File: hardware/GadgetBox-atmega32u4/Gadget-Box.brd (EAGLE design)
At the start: 93.5 x 53.5 mm, 44 parts, among them U1 MCP73831T-2ACI/OT, U2 AP2112-3.3, U3 ATMEGA32U4-XUAU, U4 ATMEGA32U4-XUMU, X1 CRYSTAL-0500290P1, X100 JSTPH

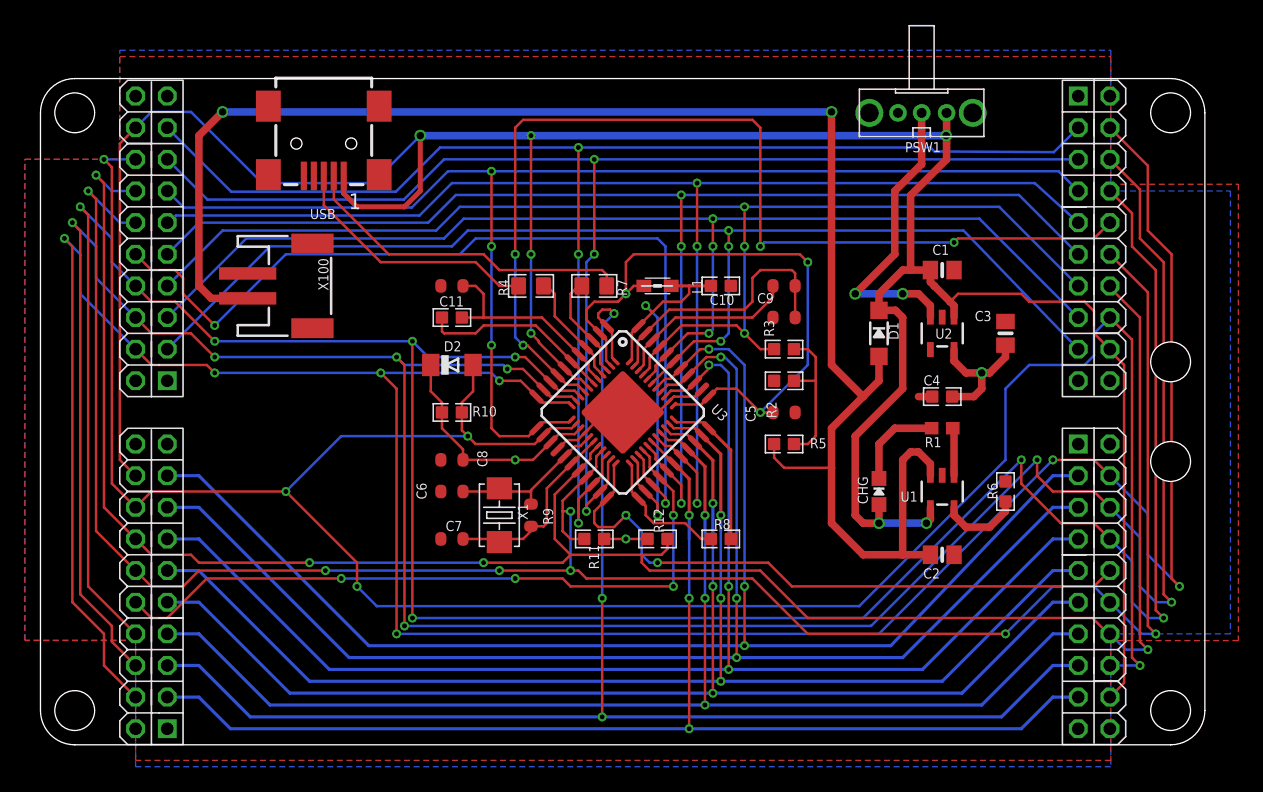
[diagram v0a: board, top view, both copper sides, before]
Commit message: cleaned up drc
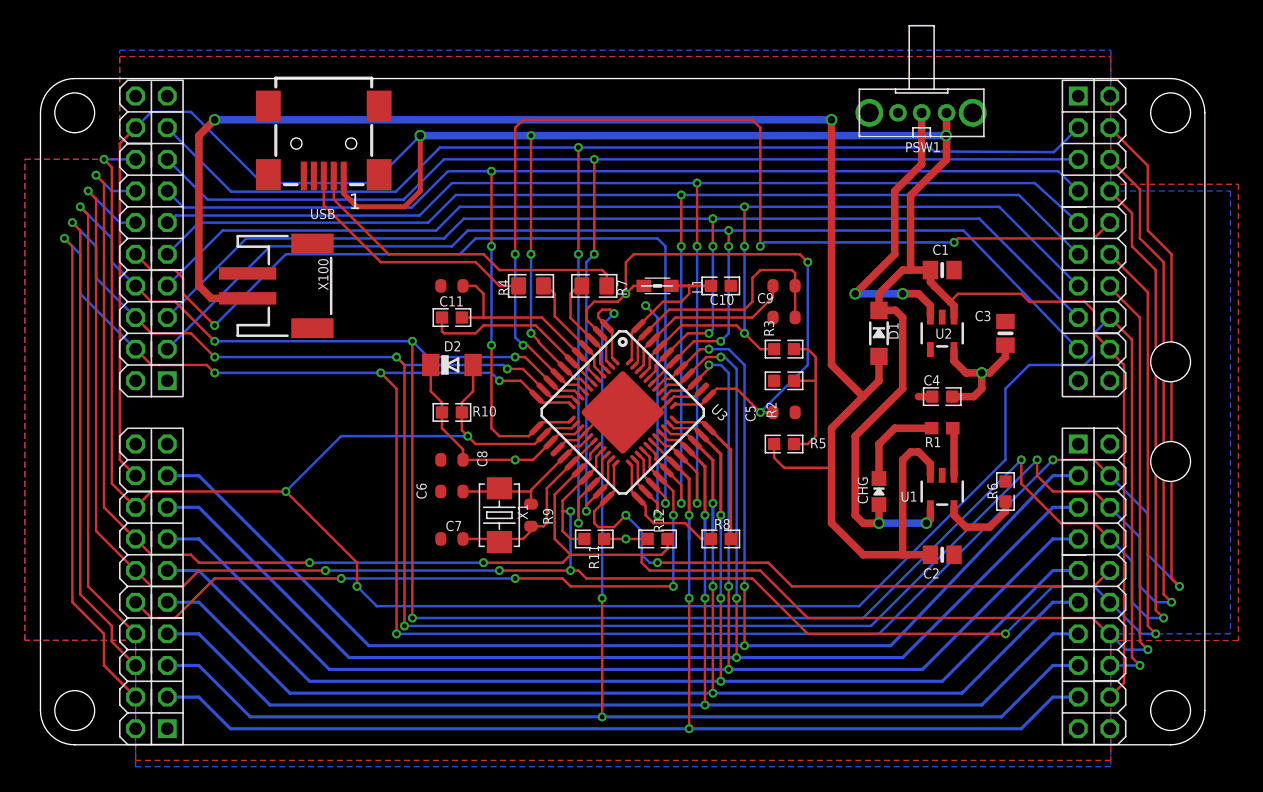
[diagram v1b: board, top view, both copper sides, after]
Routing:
- net VBAT: track 133.3 -> 132.4 mm
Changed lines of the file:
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@@
 <wire x1="50.975846875" y1="22.707409375" x2="50.165" y2="23.51825625" width="0.2032" layer="1"/>
 <wire x1="8.89" y1="12.7" x2="10.16" y2="11.43" width="0.2032" layer="1"/>
-<wire x1="10.16" y1="11.43" x2="11.43" y2="11.43" width="0.2032" layer="1"/>
-<wire x1="11.43" y1="11.43" x2="14.605" y2="14.605" width="0.2032" layer="1"/>
-<wire x1="14.605" y1="14.605" x2="25.4" y2="14.605" width="0.2032" layer="1"/>
+<wire x1="10.16" y1="11.43" x2="12.065" y2="11.43" width="0.2032" layer="1"/>
+<wire x1="12.065" y1="11.43" x2="15.24" y2="14.605" width="0.2032" layer="1"/>
+<wire x1="15.24" y1="14.605" x2="25.4" y2="14.605" width="0.2032" layer="1"/>
 <wire x1="39.37" y1="14.605" x2="43.18" y2="14.605" width="0.2032" layer="1"/>
 <wire x1="43.18" y1="14.605" x2="43.815" y2="13.97" width="0.2032" layer="1"/>
@@
 <wire x1="14.97" y1="37.1" x2="13.97" y2="38.1" width="0.6096" layer="1"/>
 <wire x1="13.97" y1="38.1" x2="13.97" y2="50.165" width="0.6096" layer="1"/>
-<wire x1="13.97" y1="50.165" x2="15.875" y2="52.07" width="0.6096" layer="1"/>
-<via x="15.875" y="52.07" extent="1-16" drill="0.6"/>
-<wire x1="15.875" y1="52.07" x2="64.77" y2="52.07" width="0.6096" layer="16"/>
-<via x="64.77" y="52.07" extent="1-16" drill="0.6"/>
-<wire x1="64.77" y1="52.07" x2="64.77" y2="31.75" width="0.6096" layer="1"/>
+<wire x1="13.97" y1="50.165" x2="15.24" y2="51.435" width="0.6096" layer="1"/>
+<via x="15.24" y="51.435" extent="1-16" drill="0.6"/>
+<wire x1="15.24" y1="51.435" x2="64.77" y2="51.435" width="0.6096" layer="16"/>
+<via x="64.77" y="51.435" extent="1-16" drill="0.6"/>
+<wire x1="64.77" y1="51.435" x2="64.77" y2="31.75" width="0.6096" layer="1"/>
 <wire x1="64.77" y1="31.75" x2="67.31" y2="29.21" width="0.6096" layer="1"/>
 <wire x1="60.16" y1="25.4" x2="60.16" y2="24.295" width="0.2032" layer="1"/>
